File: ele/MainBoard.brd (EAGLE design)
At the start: 136.6 x 100 mm, 116 parts, among them IC1 MCP23017SP, IC2 74HC595D, IC3 74HC595D, X1 POWER_IN, X2 POWER_OUT

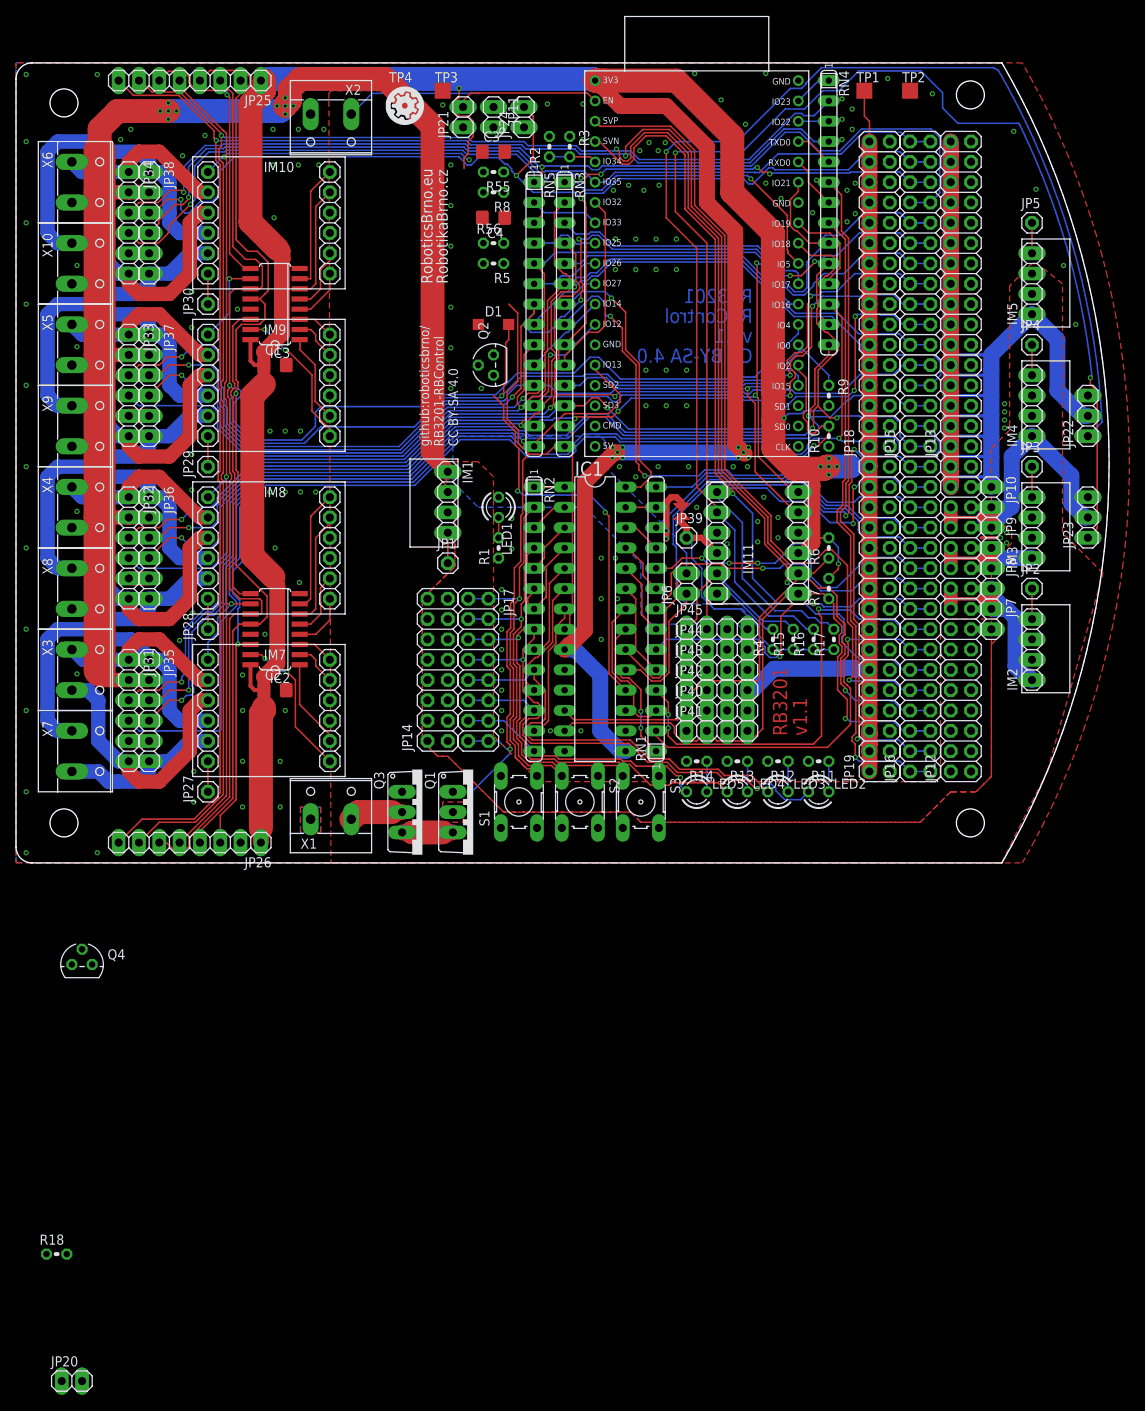
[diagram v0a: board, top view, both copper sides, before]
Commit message: ele: Finish routing v1.1
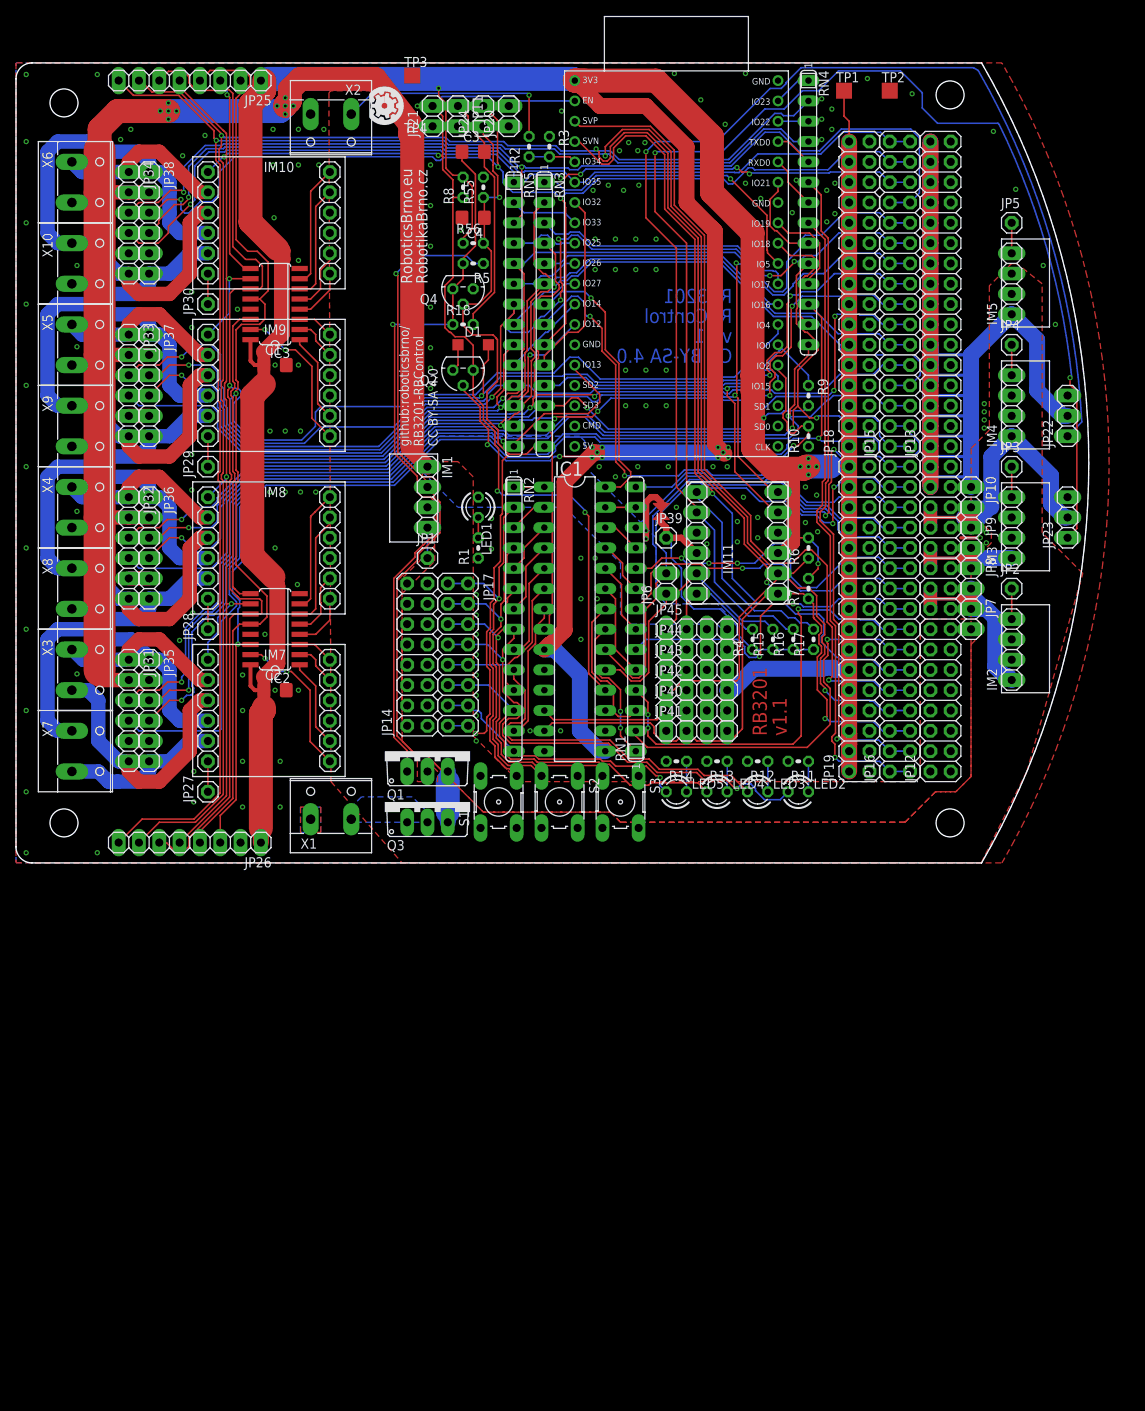
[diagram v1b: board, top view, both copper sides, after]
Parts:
- moved JP20 167.3 mm to (61.6, 93.3), turned to 90 degrees
- moved R18 126.8 mm to (55.9, 67.3)
- moved Q4 97.0 mm to (55.9, 71.8), turned to 180 degrees
- moved Q1 9.52 mm to (51.4, 14.0), turned to 0 degrees
- moved TP4 6.63 mm to (49.5, 90.2)
- moved JP24 5.08 mm to (58.4, 93.3)
- moved JP11 4.45 mm to (55.2, 93.3)
- moved TP3 4.26 mm to (49.5, 98.4)
- moved R8 3.86 mm to (55.9, 84.5), turned to 90 degrees
- moved Q2 3.86 mm to (55.9, 61.6), turned to 180 degrees
- moved JP21 3.81 mm to (52.1, 93.3)
- moved D1 3.59 mm to (57.1, 64.8)
- moved JP14 3.18 mm to (50.2, 26.0)
- moved JP17 3.18 mm to (55.2, 26.0)
- moved IM1 2.62 mm to (52.7, 50.8)
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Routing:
- net N$1: track 0.00 -> 92.7 mm, vias 0 -> 1
- net BAT_PROT: track 6.35 -> 89.9 mm, vias 0 -> 1
- net EN: track 228.1 -> 265.8 mm
- net N$6: track 0.00 -> 30.3 mm
- net +3V3: track 512.9 -> 542.5 mm, vias 18 -> 20
- net ESP_!SHUTDOWN: track 77.3 -> 101.4 mm, vias 1 -> 2
- net VCC: track 17.1 -> 28.6 mm, vias 0 -> 1
- net BAT: track 6.72 -> 0.00 mm
- net RCKMOT: track 216.6 -> 211.5 mm
- net +5V: track 208.9 -> 204.7 mm
- net ENC8A: track 140.8 -> 136.8 mm
- net _EN_: track 0.00 -> 3.44 mm
- net ENC1A: track 154.0 -> 151.5 mm
- net SCL: track 345.0 -> 342.4 mm
- net ENC6B: track 135.4 -> 132.9 mm
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- added copper zone on layer 16, net BAT
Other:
- board size 136.6 x 100 mm -> 134.1 x 100 mm
- board text added: "+5V"
- board text added: "ESP !SHDN"
- board text removed: "ESP !SHUTDOWN"
